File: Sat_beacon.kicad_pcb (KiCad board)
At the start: 2 copper layers, 3.6 x 8 mm, 126 parts, among them IC1 LMX2581ESQE_NOPB, IC2 LMX2581ESQE_NOPB, J1 Conn_01x05_Pin, J2 Conn_01x05_Pin, J3 Conn_01x03_Pin, J4 MMCX, J5 MMCX, Q1 BC817-40, Q2 BC817-40, Q3 BC817-40, Q4 BC817-40, SW1 B1407, SW2 SW_Omron_B3FS, SW3 SW_Omron_B3FS, SW4 SW_Omron_B3FS, SW5 SW_Omron_B3FS, U1 LD1117DT33, U2 LD1117DT33, U3 LD1117DT33, U4 1720BL15B0050002E, U5 1720BL15B0050002E, U7 STM32C031C6Tx, Y1 FT2MHUPM10.0-T1

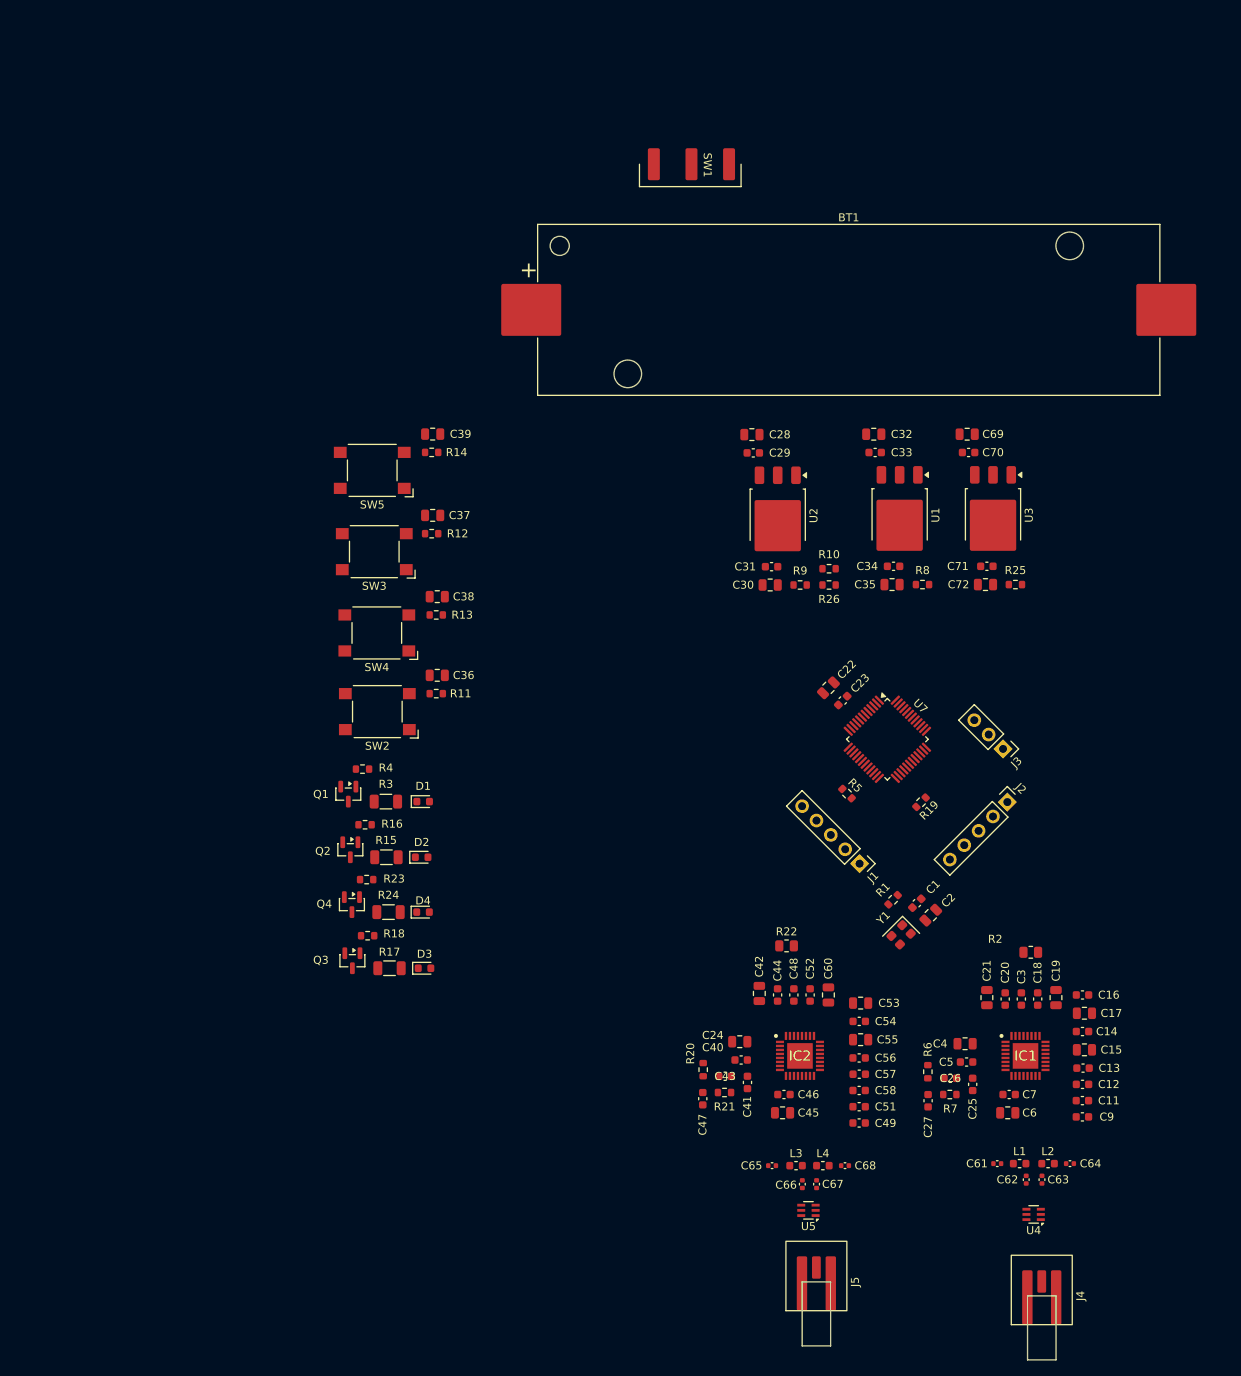
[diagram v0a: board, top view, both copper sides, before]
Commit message: PCB work
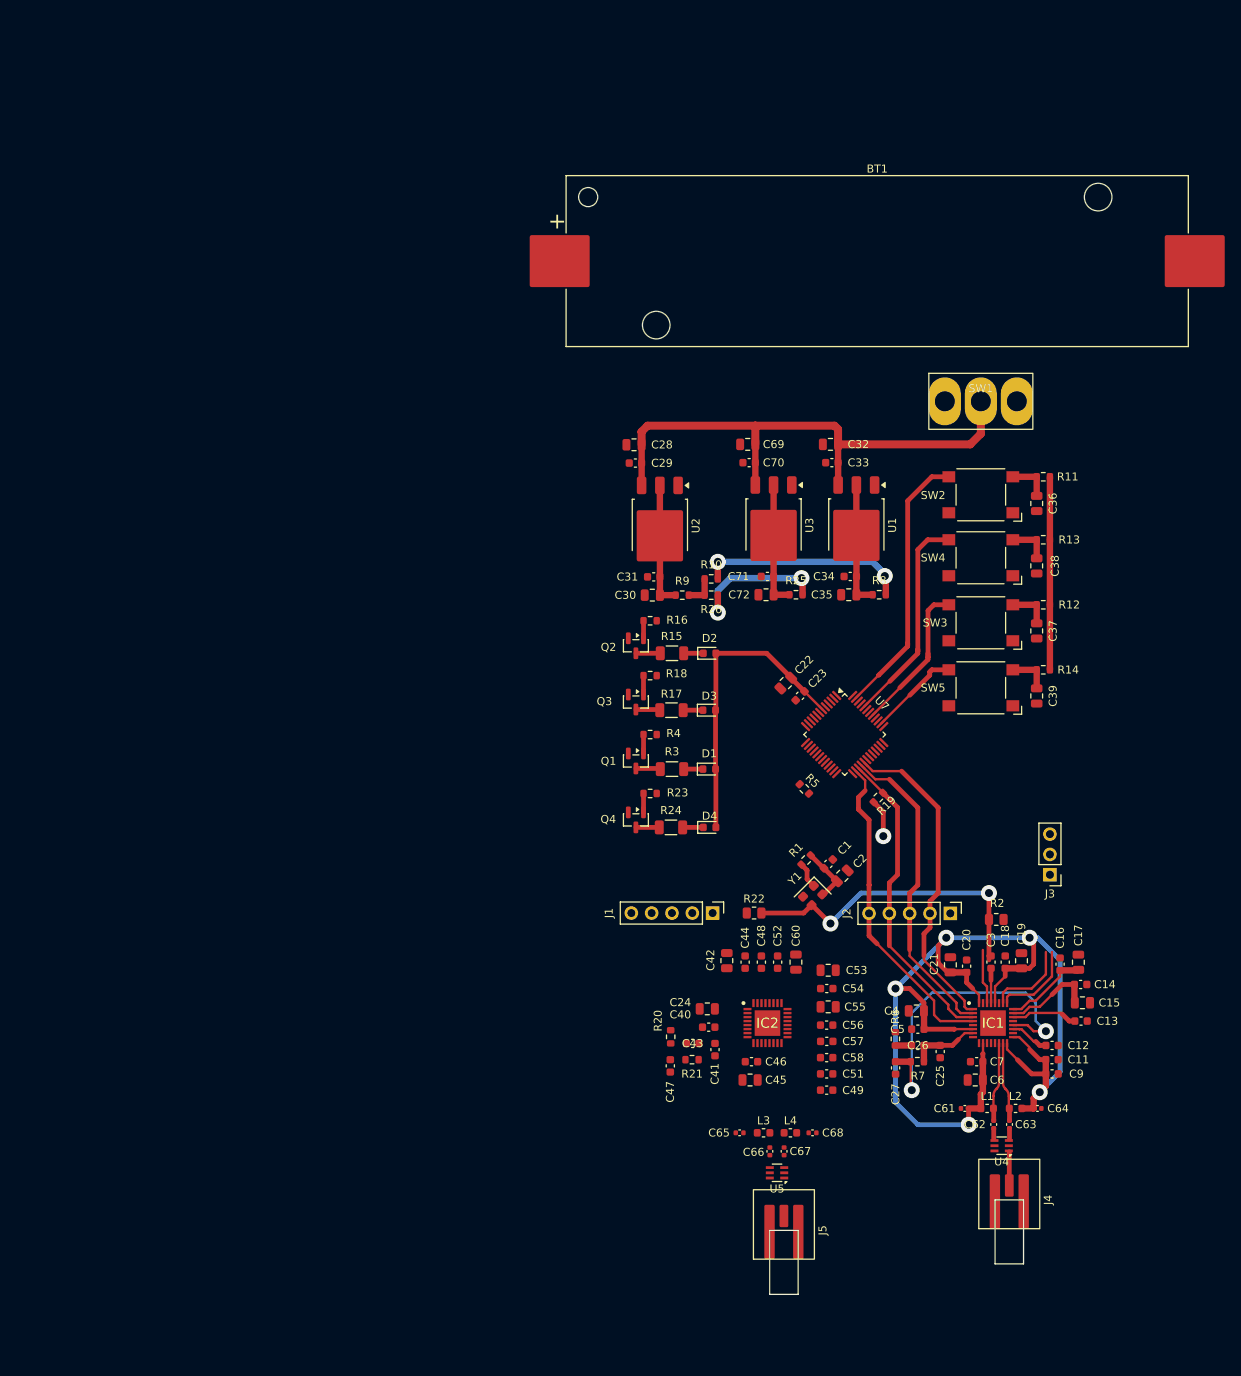
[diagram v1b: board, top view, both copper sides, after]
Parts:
- SW1: footprint Switch_sideways:B1407 -> Switch_sideways:flip_switch
- moved C39 82.3 mm to (126.4, 85.6), turned to 90 degrees
- moved R14 81.1 mm to (127.2, 82.3)
- moved SW5 80.8 mm to (119.4, 84.6)
- moved R11 80.6 mm to (127.2, 58.2)
- moved SW2 80.2 mm to (119.4, 60.5)
- moved C36 78.0 mm to (126.4, 61.5), turned to 90 degrees
- moved R12 77.0 mm to (127.2, 74.2)
- moved C37 76.9 mm to (126.4, 77.5), turned to 90 degrees
- moved R13 76.5 mm to (127.2, 66.1)
- moved SW3 76.3 mm to (119.4, 76.5)
- moved SW4 76.1 mm to (119.4, 68.3)
- moved C38 75.0 mm to (126.4, 69.3), turned to 90 degrees
- moved D3 48.0 mm to (85.4, 87.4)
- moved R18 48.0 mm to (78.0, 83.1)
- moved Q3 48.0 mm to (76.3, 86.4)
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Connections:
- SW1 pad 3: VCC_CHARGER -> +BATT
- U7 pad 10: unconnected-(U7-PF2-Pad10) -> /NRST
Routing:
- net VCC_PLL1: track 0.00 -> 163.1 mm, vias 0 -> 7
- net VCC_MCU: track 0.00 -> 78.1 mm, vias 0 -> 1
- net Net-(SW1-B): track 0.00 -> 68.6 mm
- net /VTUNE_1: track 0.00 -> 40.7 mm, vias 0 -> 2
- net /PLL_CLK_1: track 0.00 -> 40.5 mm
- net /PLL_CE_1: track 0.00 -> 40.5 mm
- net /CLK_10MHZ: track 0.00 -> 39.8 mm, vias 0 -> 2
- net /PLL_DATA_1: track 0.00 -> 39.6 mm
- net /PLL_BTN_1: track 0.00 -> 39.4 mm
- net /PLL_LE_1: track 0.00 -> 39.1 mm
- net /PLL_TOGGLE_1: track 0.00 -> 32.4 mm
- net /PLL_BTN_2: track 0.00 -> 24.7 mm
- net VCC_PLL2: track 0.00 -> 18.2 mm, vias 0 -> 2
- net /PLL_TOGGLE_2: track 0.00 -> 16.8 mm
- net Net-(U1-VO): track 0.00 -> 15.8 mm
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
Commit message: PCB work + MCU pin moves
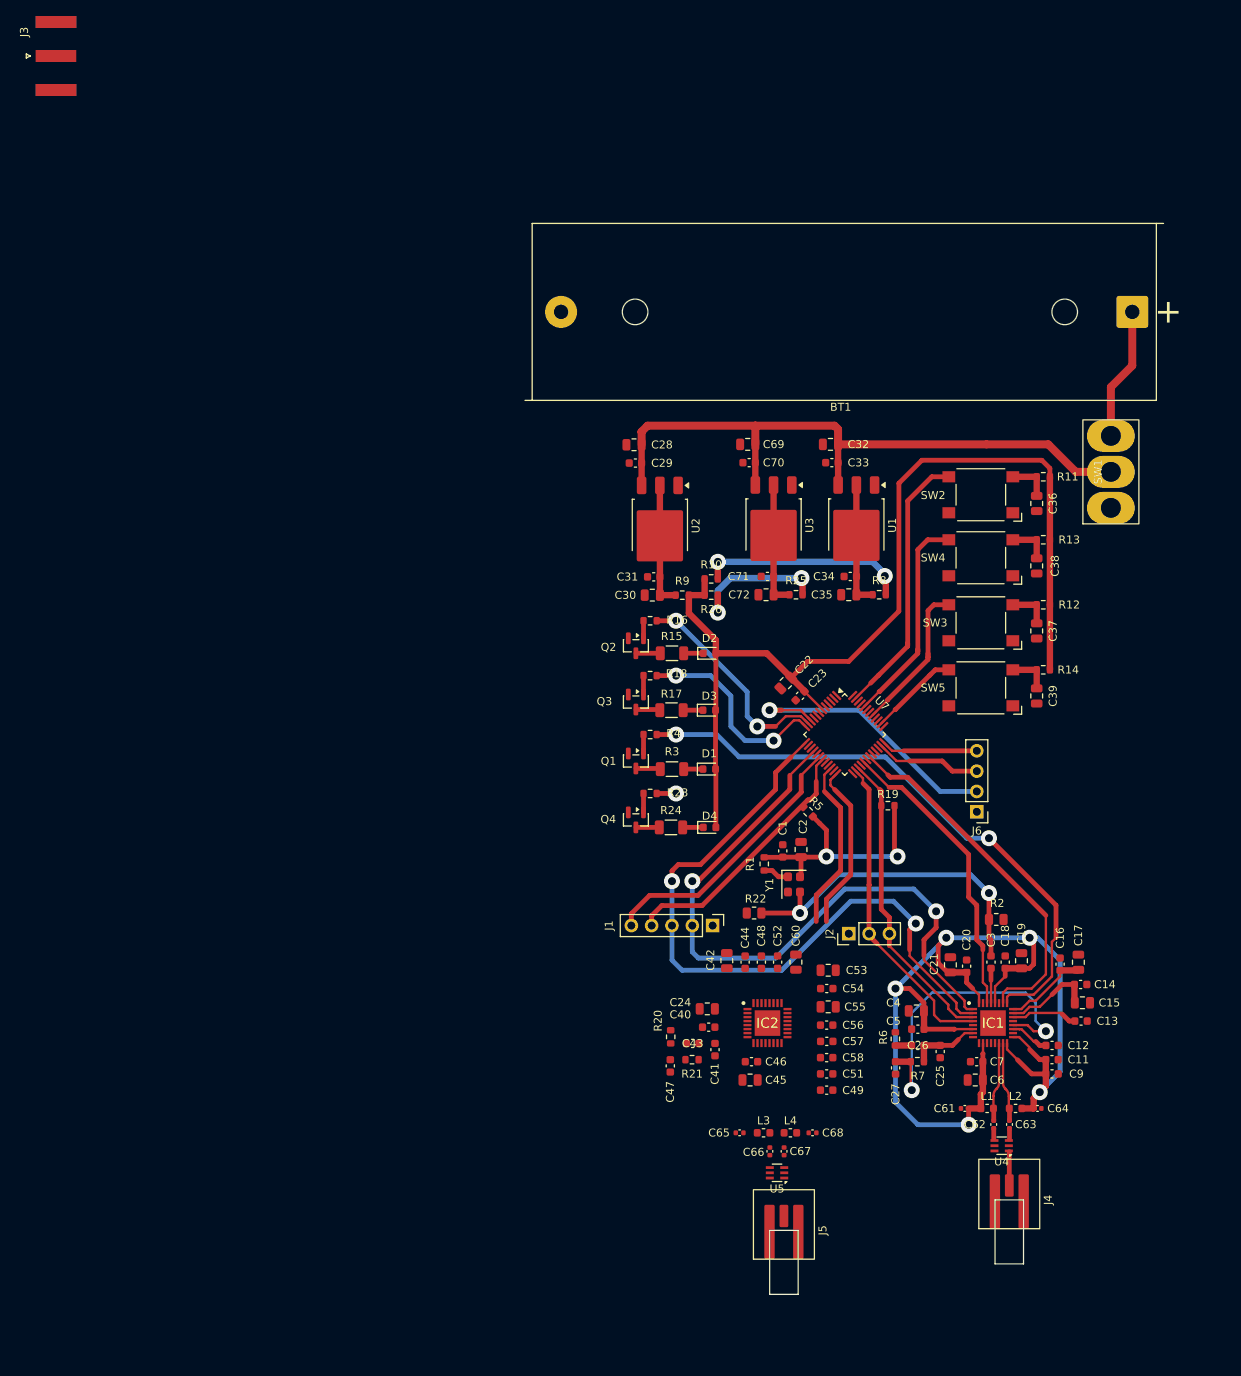
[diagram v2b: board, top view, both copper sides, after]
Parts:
- added J6: Conn_01x04_Pin, Connector_PinHeader_2.54mm:PinHeader_1x04_P2.54mm_Vertical, F.Cu at (118.9, 100.1)
- BT1: footprint Battery:BatteryHolder_Keystone_1042_1x18650 -> Battery:BatteryHolder_MPD_BH-18650-PC
- J2: value Conn_01x05_Pin -> Conn_01x03_Pin; footprint Connector_PinHeader_2.54mm:PinHeader_1x05_P2.54mm_Vertical -> Connector_PinHeader_2.54mm:PinHeader_1x03_P2.54mm_Vertical
- J3: value Conn_01x03_Pin -> Conn_Coaxial; footprint Connector_PinHeader_2.54mm:PinHeader_1x03_P2.54mm_Vertical -> Connector_Coaxial:SMA_Amphenol_132289_EdgeMount
- moved J3 161.0 mm to (3.77, 5.61), turned to 0 degrees
- moved BT1 32.5 mm to (138.3, 37.6), turned to 180 degrees
- moved SW1 18.5 mm to (135.6, 57.6), turned to 90 degrees
- moved J2 12.9 mm to (102.9, 115.3), turned to 90 degrees
- moved C2 6.12 mm to (96.9, 104.8), turned to -90 degrees
- moved C1 5.93 mm to (94.6, 105.0), turned to -90 degrees
- moved R1 5.26 mm to (92.3, 106.6), turned to -90 degrees
- moved R5 2.90 mm to (97.8, 100.1)
- moved Y1 2.72 mm to (96.0, 109.2), turned to -90 degrees
- moved R19 1.57 mm to (107.8, 99.3), turned to 0 degrees
- moved J1 1.56 mm to (85.9, 114.3)
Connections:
- IC1 pad 1: /PLL_CLK_1 -> /PLL_CLK
- IC1 pad 2: /PLL_DATA_1 -> /PLL_DATA
- IC2 pad 1: /PLL_CLK_2 -> /PLL_CLK
- IC2 pad 2: /PLL_DATA_2 -> /PLL_DATA
- J1 pad 2: /PLL_CLK_2 -> /PLL_CLK
- J1 pad 3: /PLL_DATA_2 -> /PLL_DATA
- J2 pad 2: /PLL_CLK_1 -> /PLL_CE_1
- J2 pad 3: /PLL_DATA_1 -> /PLL_LE_1
- J3 pad 1: GND -> unconnected-(J3-In-Pad1)
- J3 pad 2: /SWDIO -> unconnected-(J3-Ext-Pad2)
- U7 pad 11: unconnected-(U7-PA0-Pad11) -> /PLL_LED_1
- U7 pad 12: unconnected-(U7-PA1-Pad12) -> /PLL_LED_2
- U7 pad 13: /PLL_LED_1 -> /PLL_DATA
- U7 pad 14: /PLL_LED_2 -> unconnected-(U7-PA3-Pad14)
- U7 pad 16: unconnected-(U7-PA5-Pad16) -> /PLL_CLK
- U7 pad 17: unconnected-(U7-PA6-Pad17) -> /PLL_MUXout
- U7 pad 20: /PLL_DATA_2 -> unconnected-(U7-PB1-Pad20)
- U7 pad 21: /PLL_CLK_2 -> unconnected-(U7-PB2-Pad21)
- U7 pad 22: /PLL_MUXout_2 -> /PLL_MUXOUT_2
- U7 pad 23: /PLL_RF_EN_2 -> unconnected-(U7-PB11-Pad23)
- U7 pad 24: unconnected-(U7-PB12-Pad24) -> /PLL_RF_EN_2
- U7 pad 28: /PLL_DATA_1 -> unconnected-(U7-PA8-Pad28)
- U7 pad 29: /PLL_CLK_1 -> /PLL_MUXOUT_1
- U7 pad 30: /PLL_MUXout_1 -> unconnected-(U7-PC6-Pad30)
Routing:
- net /PLL_DATA: track 0.00 -> 87.2 mm, vias 0 -> 2
- net /PLL_CLK: track 0.00 -> 84.0 mm, vias 0 -> 2
- net VCC_MCU: track 78.1 -> 160.8 mm, vias 1 -> 2
- net /LD_1: track 10.5 -> 75.3 mm, vias 0 -> 2
- net /PLL_CLK_1: track 40.5 -> 0.00 mm
- net /PLL_DATA_1: track 39.6 -> 0.00 mm
- net /NRST: track 0.00 -> 35.9 mm, vias 0 -> 1
- net /PLL_RF_EN_1: track 10.4 -> 45.2 mm
- net /PLL_CE_2: track 0.00 -> 34.4 mm
- net /PLL_LE_2: track 0.00 -> 32.7 mm
- net /PLL_MUXOUT_1: track 6.86 -> 37.4 mm
- net /PLL_LED_1: track 0.00 -> 29.2 mm, vias 0 -> 2
- net /PLL_LED_2: track 0.00 -> 25.6 mm, vias 0 -> 2
- net /PLL_MUXOUT_2: track 0.00 -> 22.7 mm
- net /PLL_RF_EN_2: track 0.00 -> 21.1 mm
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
